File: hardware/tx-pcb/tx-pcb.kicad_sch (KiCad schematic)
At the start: 67 parts, among them J1 Conn_To_J1, J2 Conn_To_J2, J3 BLIO, J4 Conn_01x05, J5 Conn_01x04, J6 PWRO, J7 Conn_01x02_Pin, SW1 BOOT0, SW2 RESET, SW3 BTN1, SW4 BTN2, SW5 BTN3, SW6 BTN4, SW7 BTN5, SW8 SW_SPDT, SW9 SW_SPDT, U1 USBLC6-2SC6, U2 STM32WB55CEUx, X1 CS11336-32M, X2 ABS07-32.768KHZ-1-T

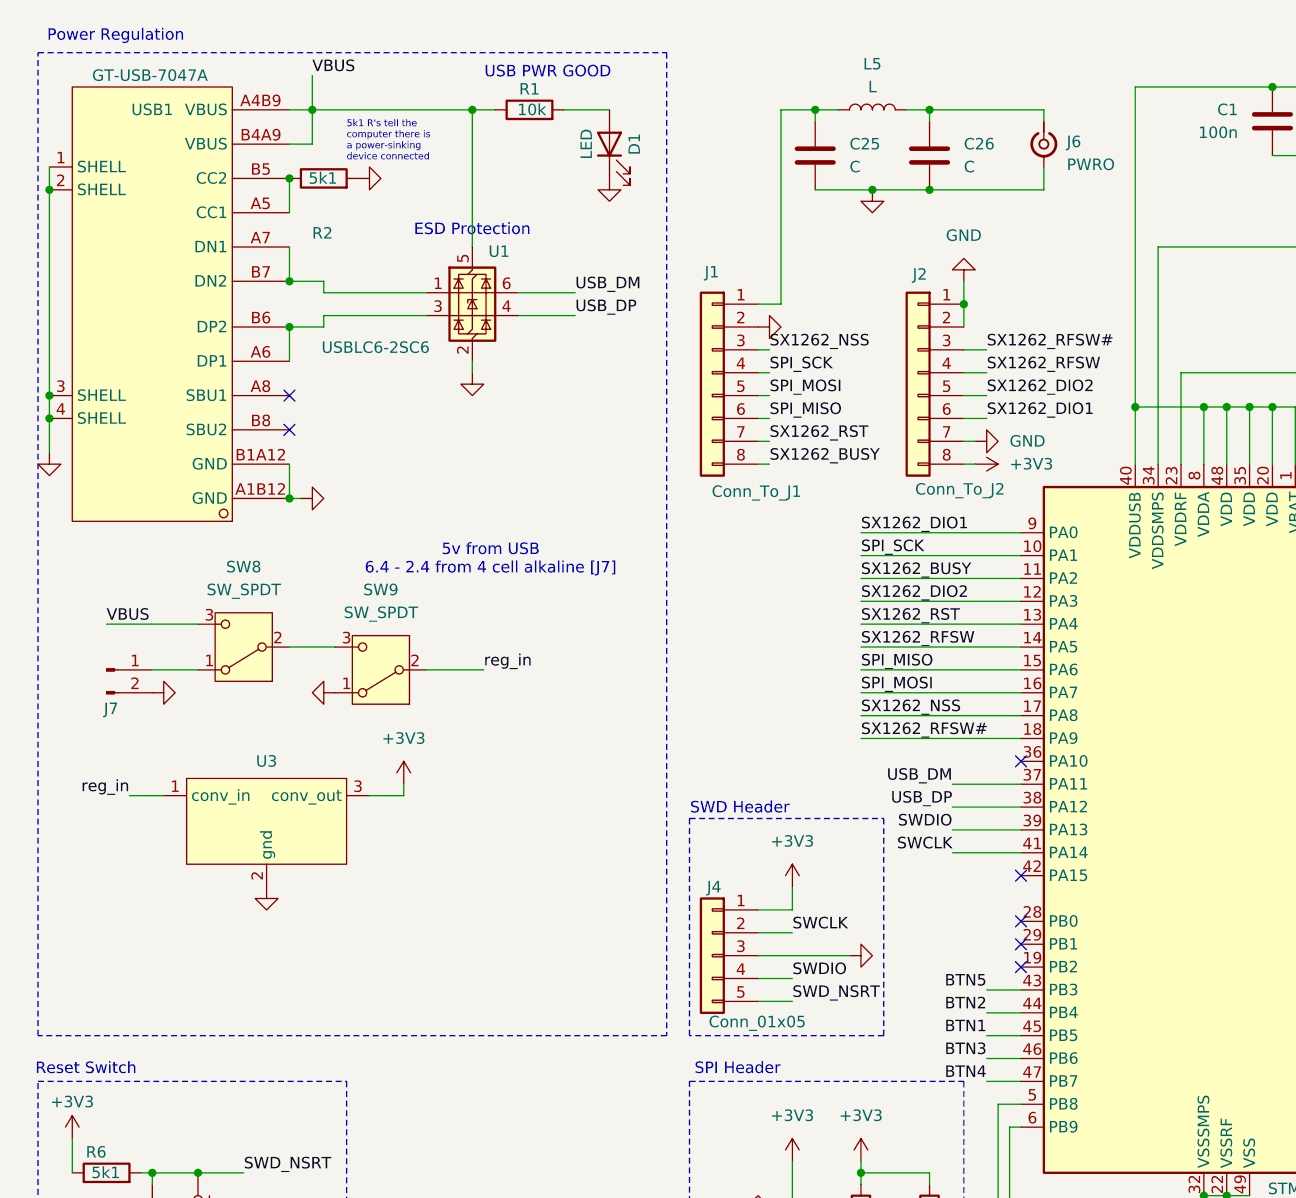
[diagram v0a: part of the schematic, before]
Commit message: updates for dr weeks
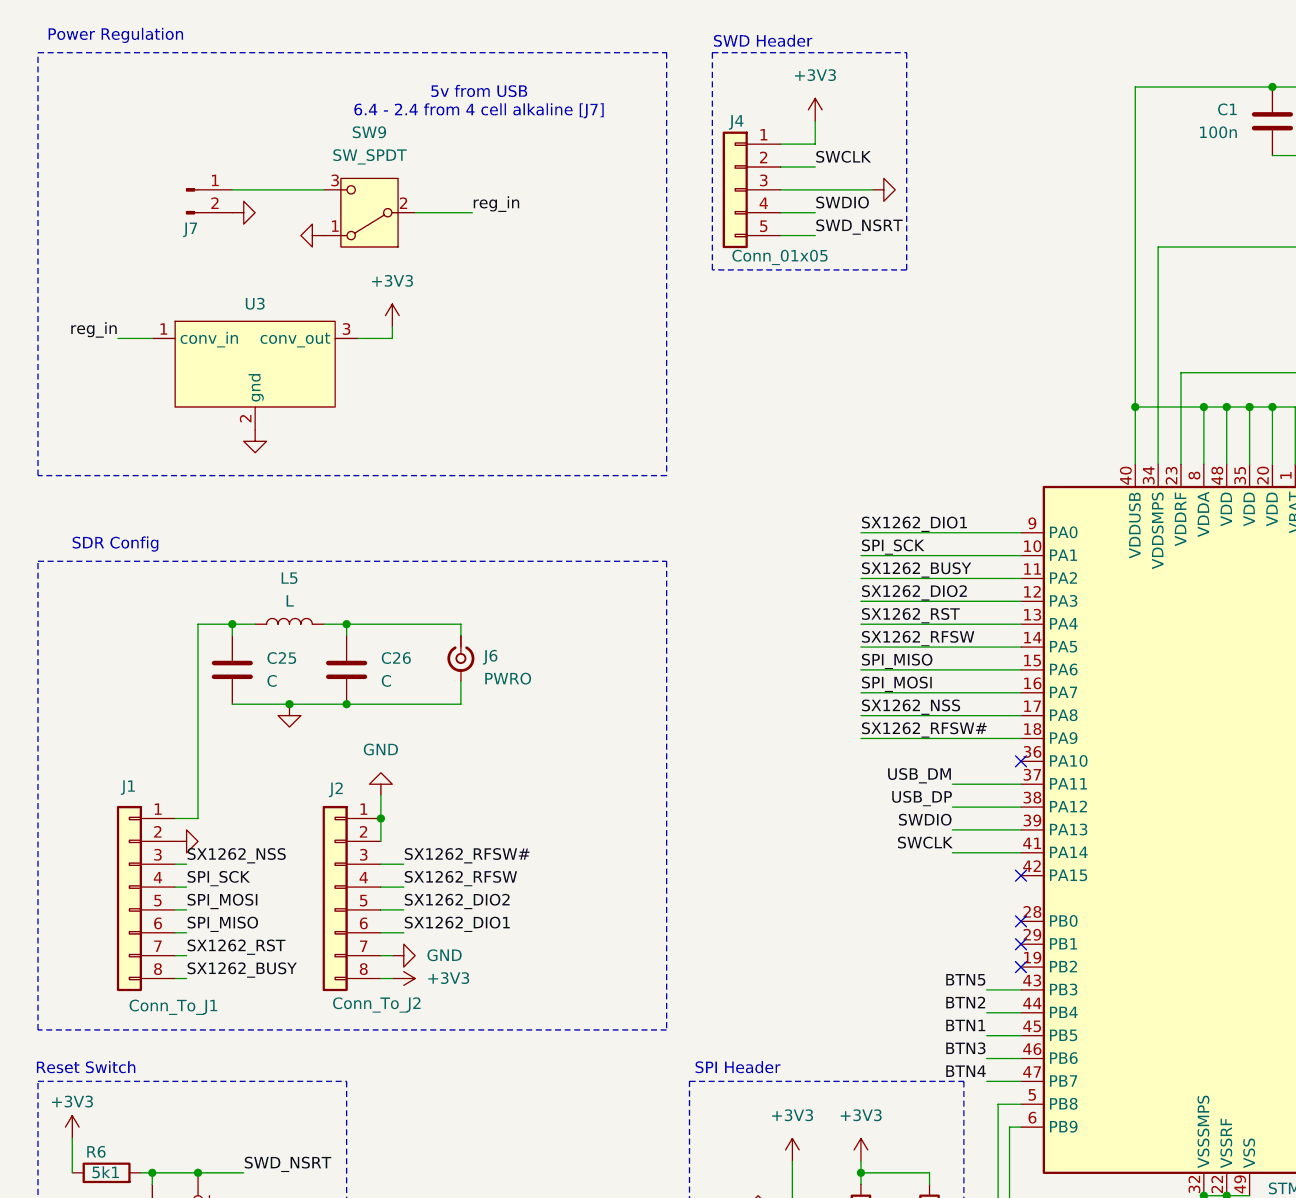
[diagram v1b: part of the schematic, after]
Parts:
- removed D1: LED, LED_SMD:LED_0603_1608Metric_Pad1.05x0.95mm_HandSolder, symbol Device:LED
- removed R1: 10k, Resistor_SMD:R_0805_2012Metric_Pad1.20x1.40mm_HandSolder, symbol Device:R
- removed R2: 5k1, Resistor_SMD:R_0805_2012Metric_Pad1.20x1.40mm_HandSolder, symbol Device:R
- removed SW8: SW_SPDT, rf-pwr-tx-library:spdt_amazon, symbol Switch:SW_SPDT
- removed U1: USBLC6-2SC6, Package_TO_SOT_SMD:SOT-23-6, symbol Power_Protection:USBLC6-2SC6
- removed USB1: GT-USB-7047A, rf-pwr-tx-library:USB-C-SMD_GT-USB-7047A, symbol rf-pwr-tx-library:GT-USB-7047A
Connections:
- net at J7.1 (Pin_1): now also SW9.3 (C)
- no-connect marks 8 -> 6
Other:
- note added: "SDR Config"
- note removed: "5k1 R's tell the computer there is a power-sinking device connected"
- note removed: "ESD Protection"
- note removed: "USB PWR GOOD"
- moved on the sheet: C25, C26, J1, J2, J4, J6, J7, L5, SW9, U3
